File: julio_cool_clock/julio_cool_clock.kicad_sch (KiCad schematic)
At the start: 4 parts

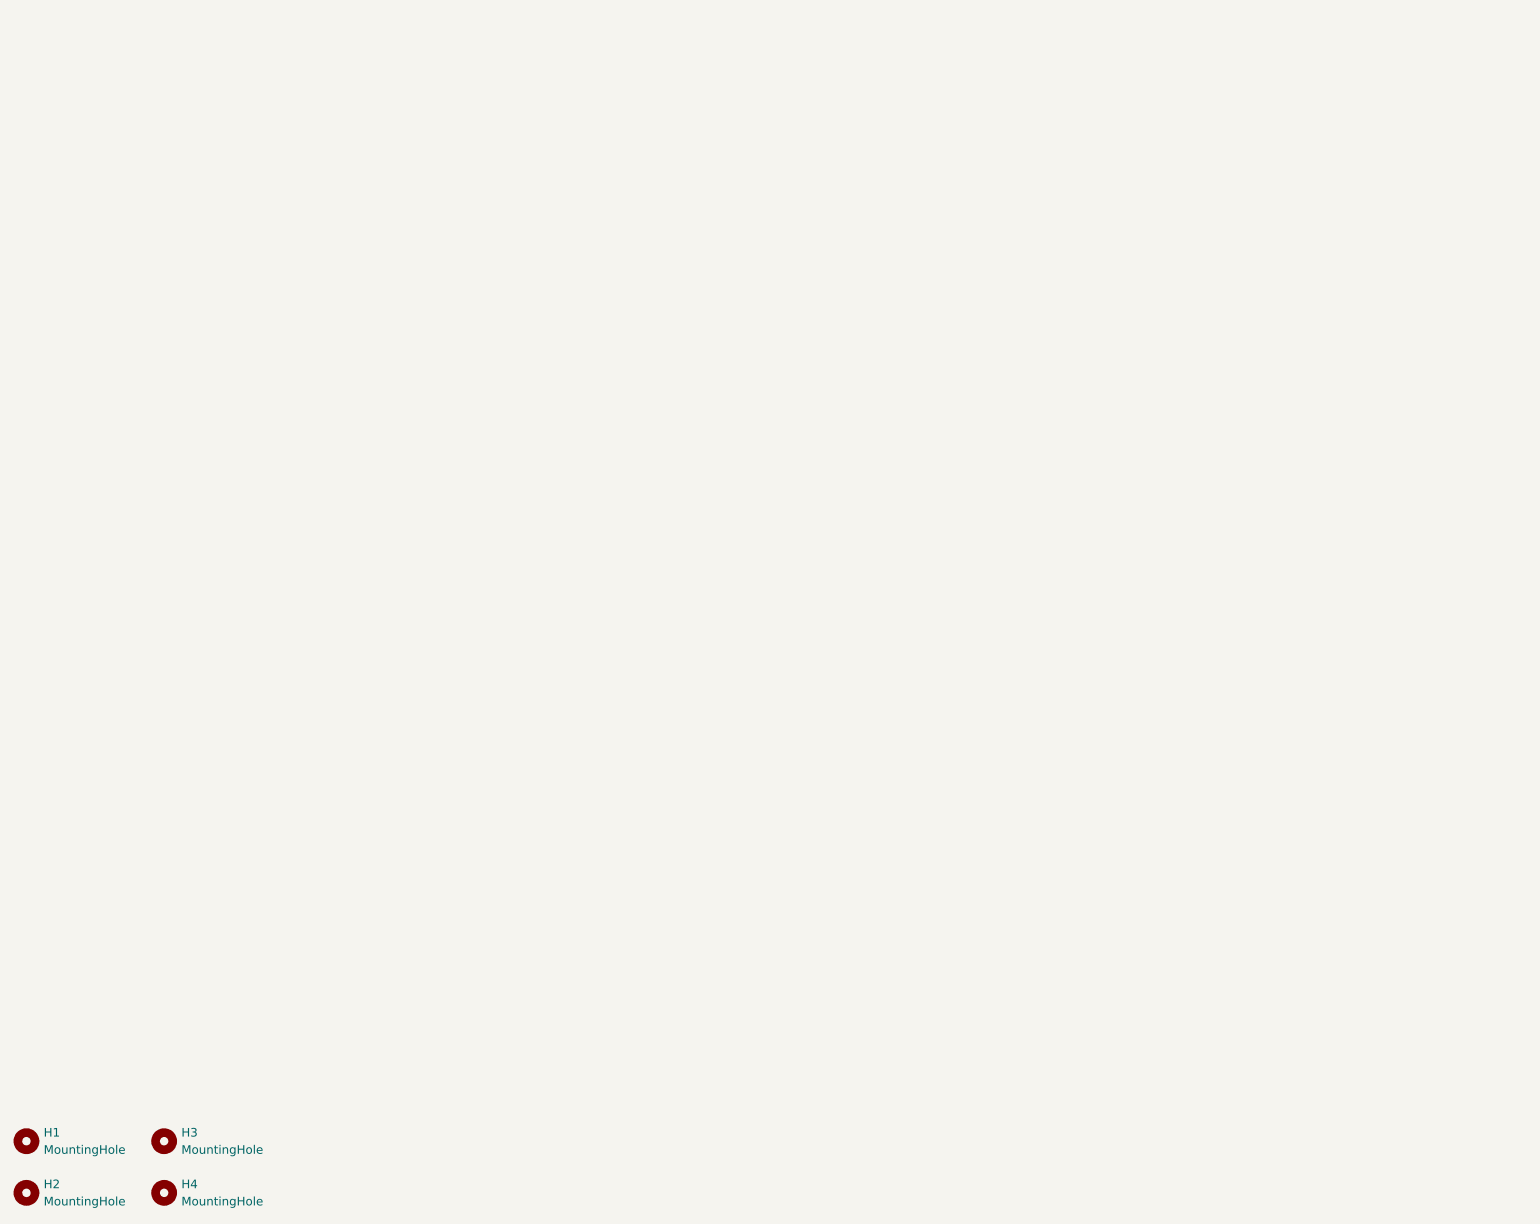
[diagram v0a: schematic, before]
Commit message: Clock Design 1
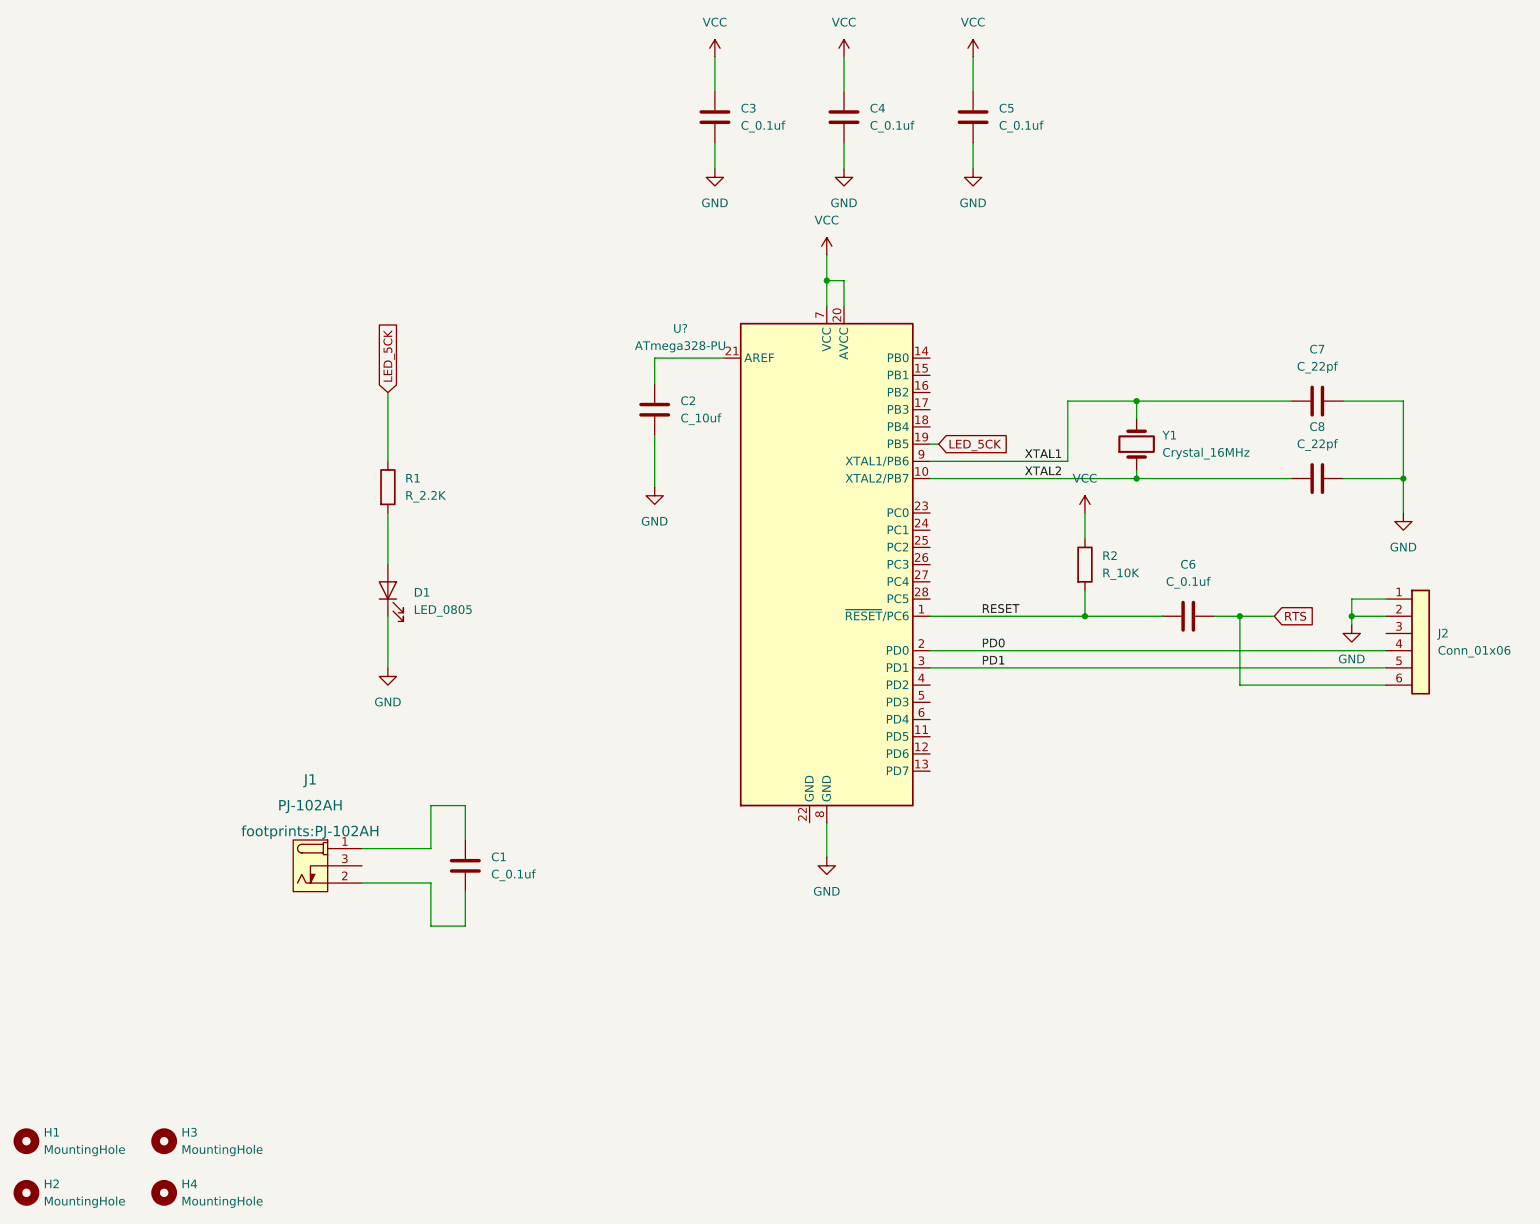
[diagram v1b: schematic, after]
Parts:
- added C1, C3, C4, C5, C6: C_0.1uf, footprints:C_0805_2012Metric, symbol HPS:C_0805_0.1uf
- added C2: C_10uf, footprints:C_0805_2012Metric, symbol HPS:C_0805_10uf
- added C7, C8: C_22pf, footprints:C_0805_2012Metric, symbol HPS:C_0805_22pf
- added D1: LED_0805, footprints:LED_0805_2012Metric, symbol HPS:LED_0805
- added J1: PJ-102AH, footprints:PJ-102AH, symbol HPS:PJ-102AH
- added J2: Conn_01x06, symbol HPS:Conn_01x06
- added R1: R_2.2K, footprints:R_0805_2012Metric, symbol HPS:R_0805_2.2K
- added R2: R_10K, footprints:R_0805_2012Metric, symbol HPS:R_0805_10K
- added U?: ATmega328-PU, footprints:DIP-28_W7.62mm, symbol HPS:ATmega328-PU
- added Y1: Crystal_16MHz, footprints:Crystal_SMD_HC49-SD, symbol HPS:Crystal_16MHz
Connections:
- new net: D1.2 (A), R1.2
- new net: C1.1, J1.1 (POLE)
- new net: C1.2, J1.2 (OUT)
- new net: C2.1, U?.21 (AREF)
- new net GND: C2.2, C3.2, C4.2, C5.2, C7.2, C8.1, D1.1 (K), J2.1 (Pin_1), J2.2 (Pin_2), U?.8 (GND)
- new net LED_5CK: R1.1, U?.19 (PB5)
- new net PD0: J2.4 (Pin_4), U?.2 (PD0)
- new net PD1: J2.5 (Pin_5), U?.3 (PD1)
- new net RESET: C6.1, R2.2, U?.1 (~{RESET}/PC6)
- new net RTS: C6.2, J2.6 (Pin_6)
- new net VCC: C3.1, C4.1, C5.1, R2.1, U?.20 (AVCC), U?.7 (VCC)
- new net XTAL1: C7.1, U?.9 (XTAL1/PB6), Y1.2
- new net XTAL2: C8.2, U?.10 (XTAL2/PB7), Y1.1
